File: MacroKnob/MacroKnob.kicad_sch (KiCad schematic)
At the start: 6 parts, among them SW1 RotaryEncoder_Switch_MP, U2 Sparkfun_Pro_Micro

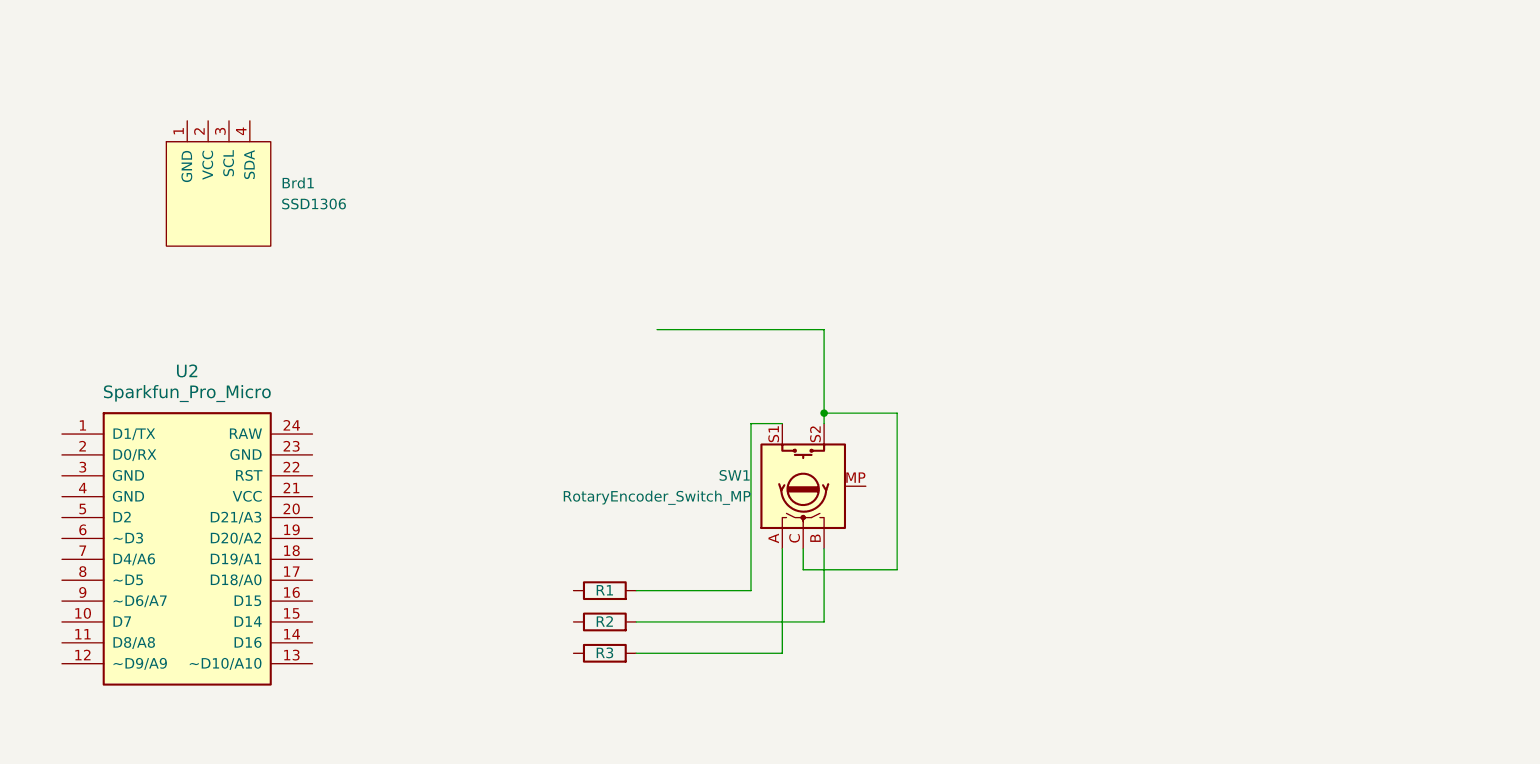
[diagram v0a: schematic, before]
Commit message: update schematic & pcb
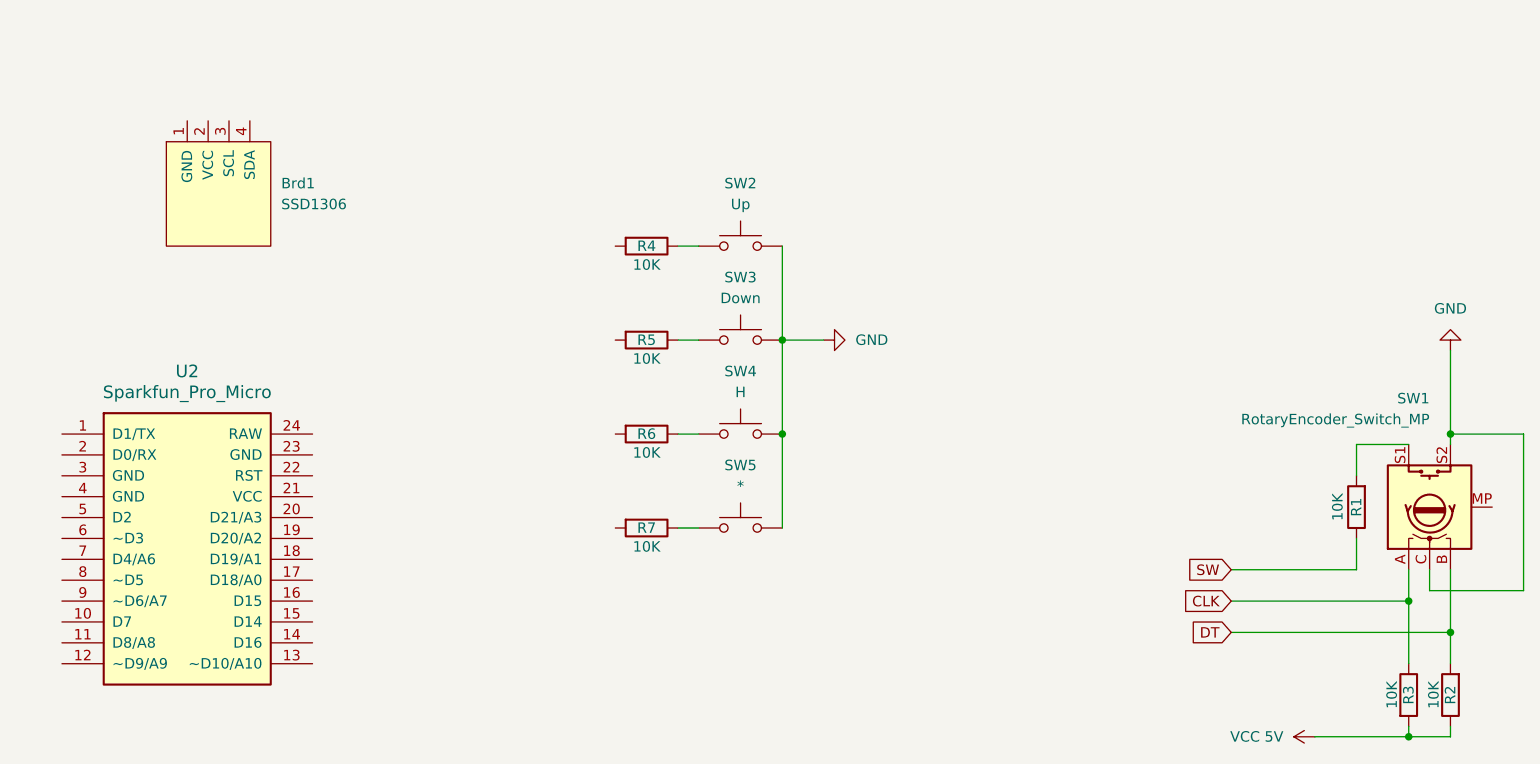
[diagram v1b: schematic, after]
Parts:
- added R4, R5, R6, R7: 10K, Resistor_THT:R_Axial_DIN0204_L3.6mm_D1.6mm_P5.08mm_Horizontal, symbol Device:R
- added SW2: Up, Button_Switch_SMD:SW_SPST_CK_RS282G05A3, symbol Switch:SW_Push
- added SW3: Down, Button_Switch_SMD:SW_SPST_CK_RS282G05A3, symbol Switch:SW_Push
- added SW4: H, Button_Switch_SMD:SW_SPST_CK_RS282G05A3, symbol Switch:SW_Push
- added SW5: *, Button_Switch_SMD:SW_SPST_CK_RS282G05A3, symbol Switch:SW_Push
- R1, R2, R3: value R -> 10K
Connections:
- net VCC 5V: now reaches R2.1
- net VCC 5V: now also R3.2
- net DT: now reaches R2.2, SW1.B
- net CLK: now reaches R3.1
- net CLK: now also SW1.A
- net GND: now reaches SW1.C, SW1.S2
- net GND: now also SW2.2, SW3.2, SW4.2, SW5.2
- net SW: now reaches R1.1
- new net: R6.1, SW4.1
- new net: R4.1, SW2.1
- new net: R5.1, SW3.1
- new net: R7.1, SW5.1
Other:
- moved on the sheet: R1, R2, R3, SW1

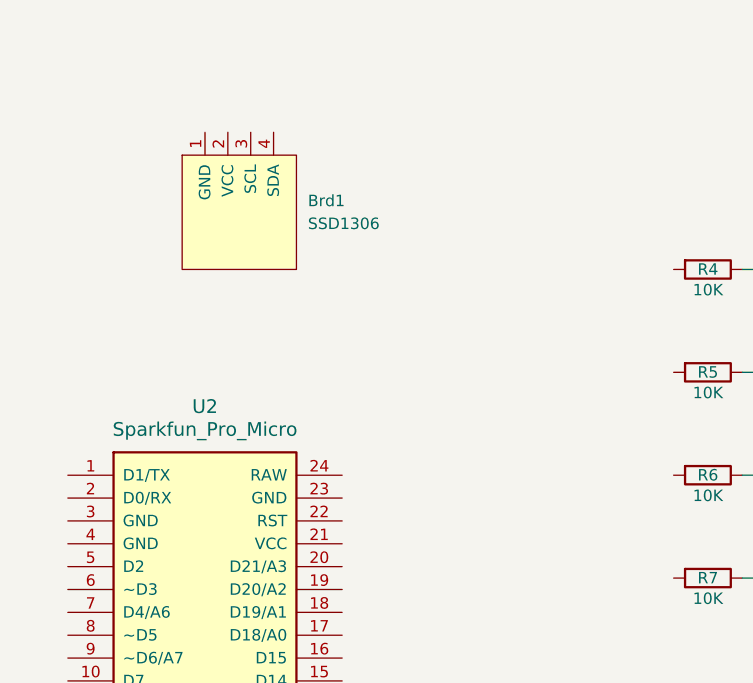
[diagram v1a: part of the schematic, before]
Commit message: update
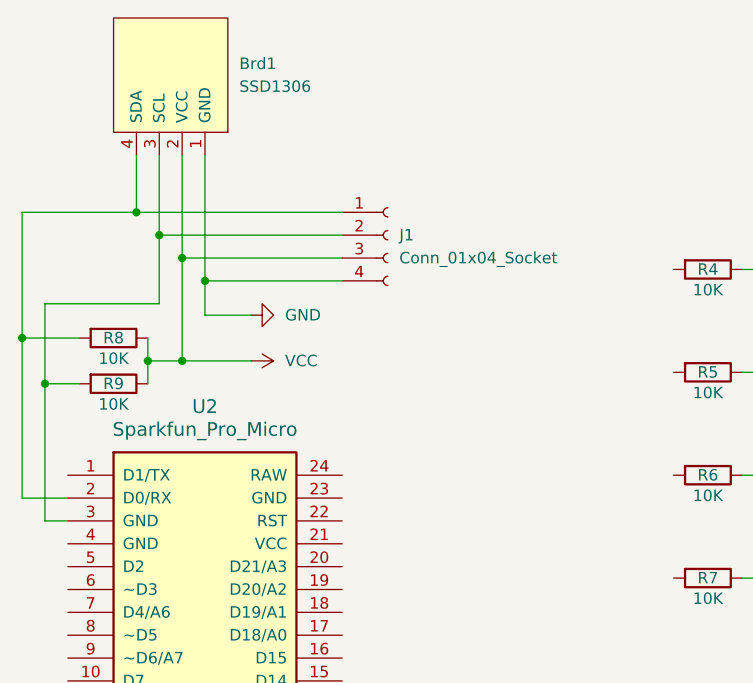
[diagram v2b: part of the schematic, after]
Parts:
- added J1: Conn_01x04_Socket, Connector_Samtec:Samtec_FMC_ASP-134486-01_10x40_P1.27mm_Vertical, symbol Connector:Conn_01x04_Socket
- added R8, R9: 10K, Resistor_THT:R_Axial_DIN0204_L3.6mm_D1.6mm_P5.08mm_Horizontal, symbol Device:R
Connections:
- net GND: now also Brd1.1 (GND), J1.4 (Pin_4)
- net VCC: now reaches Brd1.2 (VCC)
- net VCC: now also J1.3 (Pin_3), R8.1, R9.1
- net at Brd1.3 (SCL): now also U2.3 (GND), J1.2 (Pin_2), R9.2
- net at Brd1.4 (SDA): now also U2.2 (D0/RX), J1.1 (Pin_1), R8.2
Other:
- moved on the sheet: Brd1
